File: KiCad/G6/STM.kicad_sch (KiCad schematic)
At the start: 1 part, among them U16 STM32C011F4U6TR

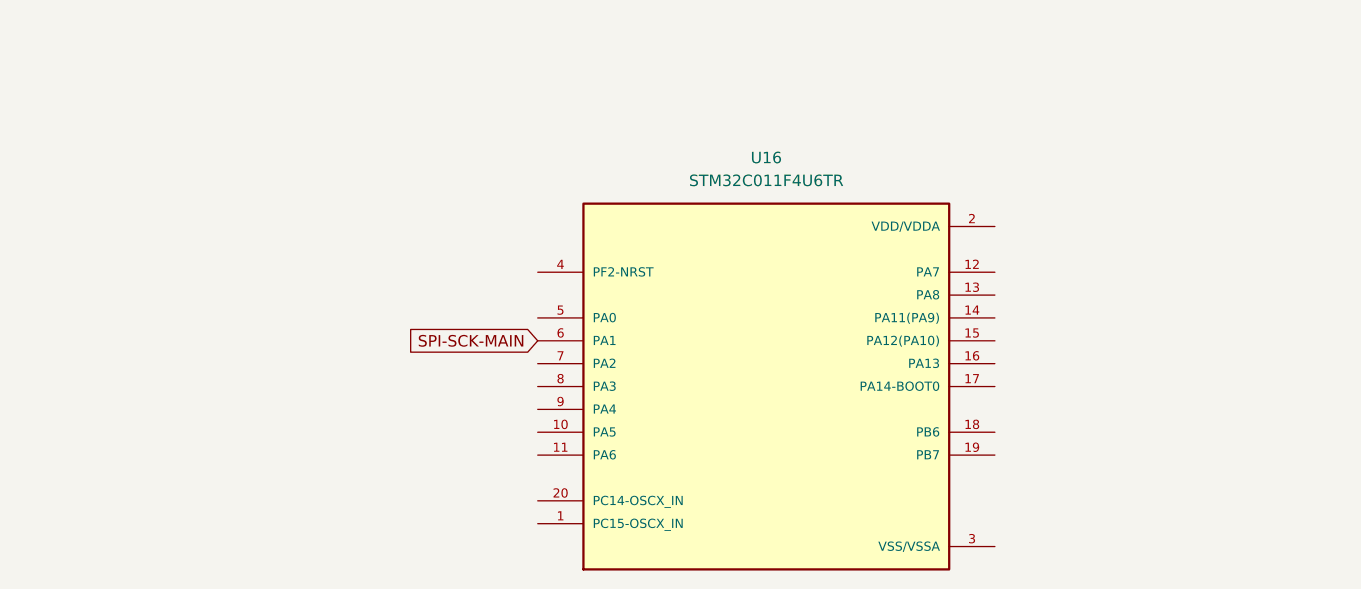
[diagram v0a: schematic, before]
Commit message: uhhhh im confused gang
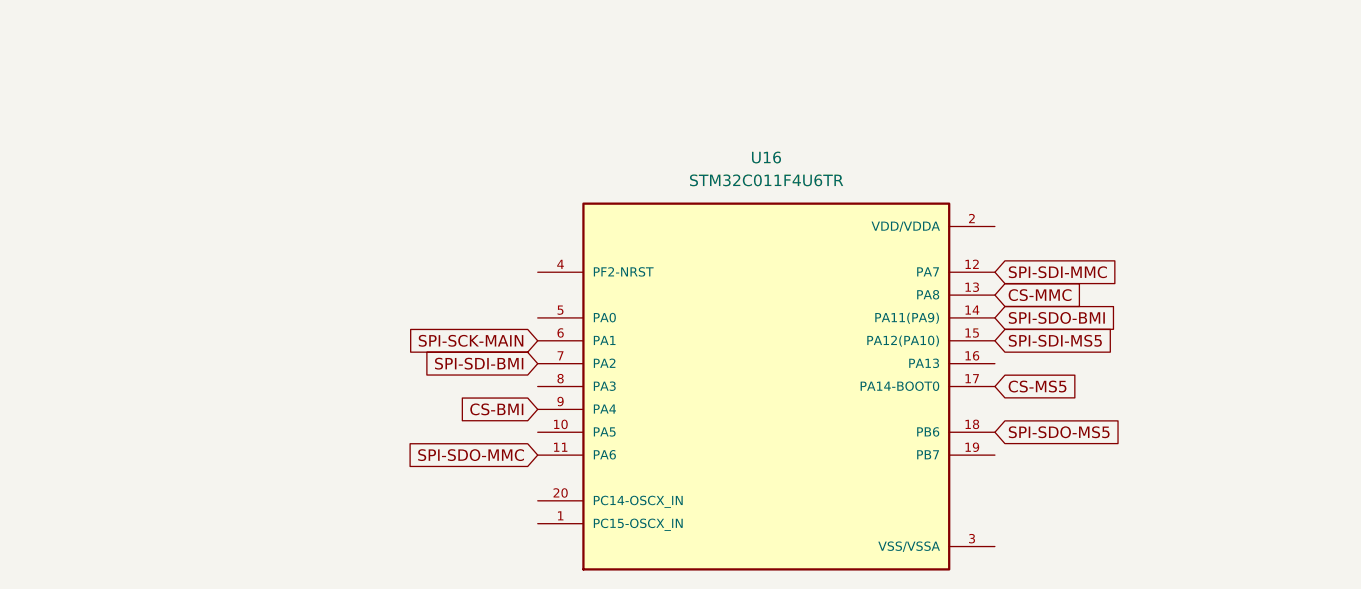
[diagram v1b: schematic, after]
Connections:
- net SPI-SDO-MMC: now reaches U16.11 (PA6)
- net SPI-SDI-MMC: now reaches U16.12 (PA7)
- net CS-MMC: now reaches U16.13 (PA8)
- net SPI-SDO-BMI: now reaches U16.14 (PA11(PA9))
- net SPI-SDI-MS5: now reaches U16.15 (PA12(PA10))
- net CS-MS5: now reaches U16.17 (PA14-BOOT0)
- net SPI-SDO-MS5: now reaches U16.18 (PB6)
- net SPI-SDI-BMI: now reaches U16.7 (PA2)
- net CS-BMI: now reaches U16.9 (PA4)
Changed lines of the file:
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@@
 	(generator_version "9.0")
 	(paper "A4")
+	(global_label "SPI-SDO-BMI"
+		(shape input)
+		(at 170.18 86.36 0)
+		(fields_autoplaced yes)
+		(effects
+			(font
+				(size 1.27 1.27)
+			)
+			(justify left)
+		)
+		(property "Intersheetrefs" "${INTERSHEET_REFS}"
+			(at 186.5305 86.36 0)
+			(effects
+				(font
+					(size 1.27 1.27)
+				)
+				(justify left)
+				(hide yes)
+			)
+		)
+	)
+	(global_label "SPI-SDI-BMI"
+		(shape input)
+		(at 119.38 91.44 180)
+		(fields_autoplaced yes)
+		(effects
+			(font
+				(size 1.27 1.27)
+			)
+			(justify right)
+		)
+		(property "Intersheetrefs" "${INTERSHEET_REFS}"
+			(at 103.7552 91.44 0)
+			(effects
+				(font
+					(size 1.27 1.27)
+				)
+				(justify right)
+				(hide yes)
+			)
+		)
+	)
 	(global_label "SPI-SCK-MAIN"
 		(shape input)
@@
 			(effects
 				(font
+					(size 1.27 1.27)
+				)
+				(justify right)
+				(hide yes)
+			)
+		)
+	)
+	(global_label "CS-MMC"
+		(shape input)
+		(at 170.18 83.82 0)
+		(fields_autoplaced yes)
+		(effects
+			(font
+				(size 1.27 1.27)
+			)
+			(justify left)
+		)
+		(property "Intersheetrefs" "${INTERSHEET_REFS}"
+			(at 181.3899 83.82 0)
+			(effects
+				(font
+					(size 1.27 1.27)
+				)
+				(justify left)
+				(hide yes)
+			)
+		)
+	)
+	(global_label "CS-BMI"
+		(shape input)
+		(at 119.38 96.52 180)
+		(fields_autoplaced yes)
+		(effects
+			(font
+				(size 1.27 1.27)
+			)
+			(justify right)
+		)
+		(property "Intersheetrefs" "${INTERSHEET_REFS}"
+			(at 109.0167 96.52 0)
+			(effects
+				(font
+					(size 1.27 1.27)
+				)
+				(justify right)
+				(hide yes)
+			)
+		)
+	)
+	(global_label "SPI-SDI-MMC"
+		(shape input)
+		(at 170.18 81.28 0)
+		(fields_autoplaced yes)
+		(effects
+			(font
+				(size 1.27 1.27)
+			)
+			(justify left)
+		)
+		(property "Intersheetrefs" "${INTERSHEET_REFS}"
+			(at 186.6514 81.28 0)
+			(effects
+				(font
+					(size 1.27 1.27)
+				)
+				(justify left)
+				(hide yes)
+			)
+		)
+	)
+	(global_label "CS-MS5"
+		(shape input)
+		(at 170.18 93.98 0)
+		(fields_autoplaced yes)
+		(effects
+			(font
+				(size 1.27 1.27)
+			)
+			(justify left)
+		)
+		(property "Intersheetrefs" "${INTERSHEET_REFS}"
+			(at 181.0875 93.98 0)
+			(effects
+				(font
+					(size 1.27 1.27)
+				)
+				(justify left)
+				(hide yes)
+			)
+		)
+	)
+	(global_label "SPI-SDI-MS5"
+		(shape input)
+		(at 170.18 88.9 0)
+		(fields_autoplaced yes)
+		(effects
+			(font
+				(size 1.27 1.27)
+			)
+			(justify left)
+		)
+		(property "Intersheetrefs" "${INTERSHEET_REFS}"
+			(at 186.349 88.9 0)
+			(effects
+				(font
+					(size 1.27 1.27)
+				)
+				(justify left)
+				(hide yes)
+			)
+		)
+	)
+	(global_label "SPI-SDO-MS5"
+		(shape input)
+		(at 170.18 99.06 0)
+		(fields_autoplaced yes)
+		(effects
+			(font
+				(size 1.27 1.27)
+			)
+			(justify left)
+		)
+		(property "Intersheetrefs" "${INTERSHEET_REFS}"
+			(at 187.0747 99.06 0)
+			(effects
+				(font
+					(size 1.27 1.27)
+				)
+				(justify left)
+				(hide yes)
+			)
+		)
+	)
+	(global_label "SPI-SDO-MMC"
+		(shape input)
+		(at 119.38 101.6 180)
+		(fields_autoplaced yes)
+		(effects
+			(font
+				(size 1.27 1.27)
+			)
+			(justify right)
+		)
+		(property "Intersheetrefs" "${INTERSHEET_REFS}"
+			(at 102.1829 101.6 0)
+			(effects
+				(font

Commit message: I think the schematics done uhhh idrk
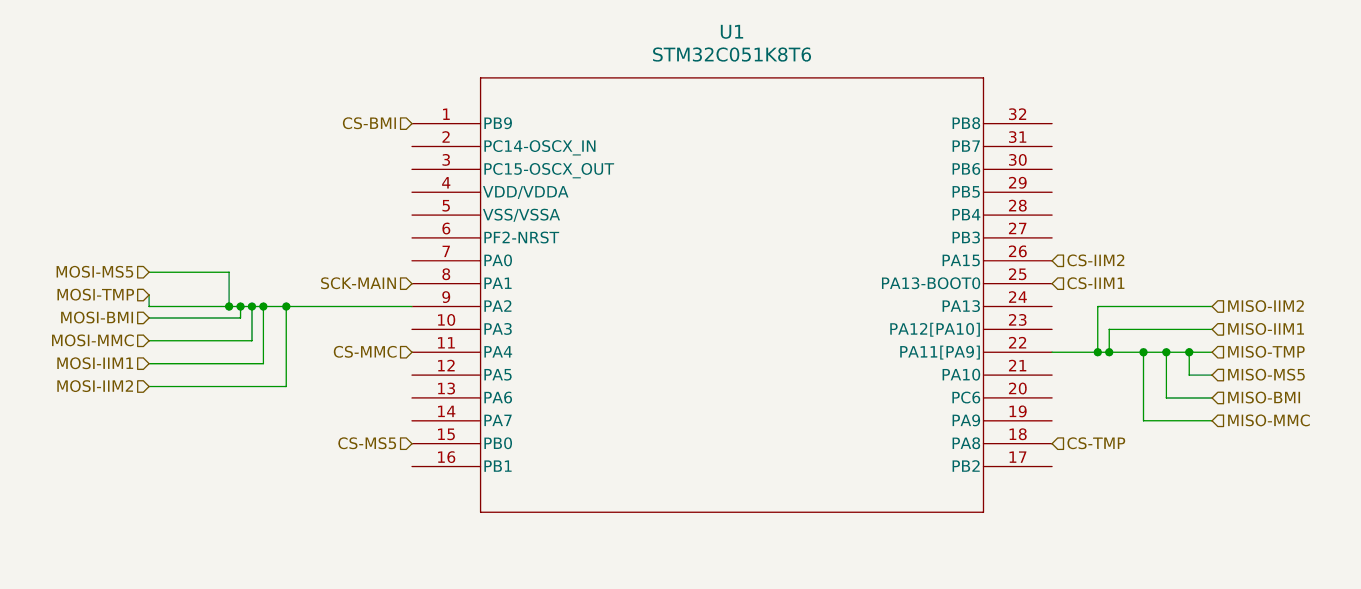
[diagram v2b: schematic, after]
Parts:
- removed U16: STM32C011F4U6TR, STM32C011F4U6TR:IC_STM32C011F4U6TR, symbol STM32C011F4U6TR:STM32C011F4U6TR
- added U1: STM32C051K8T6, CC0603KRXQRQBB104:LQFP32_7x7_STM, symbol STM32C051K8T6:STM32C051K8T6
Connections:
- net CS-BMI: now also U1.1 (PB9)
- net CS-MMC: now also U1.11 (PA4)
- net CS-MS5: now also U1.15 (PB0)
- new net CS-IIM1: U1.25 (PA13-BOOT0)
- new net CS-IIM2: U1.26 (PA15)
- new net CS-TMP: U1.18 (PA8)
- new net MISO-BMI: U1.22 (PA11[PA9])
- new net MOSI-BMI: U1.9 (PA2)
- new net SCK-MAIN: U1.8 (PA1)
